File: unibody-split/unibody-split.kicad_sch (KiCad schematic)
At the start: 103 parts, among them IC1 AP130-20, SW1 SW_Push, SW10 SW_Push, SW11 SW_Push, SW12 SW_Push, SW13 SW_Push, SW14 SW_Push, SW15 SW_Push, SW16 SW_Push, SW17 SW_Push, SW18 SW_Push, SW19 SW_Push, SW2 SW_Push, SW20 SW_Push, SW21 SW_Push, SW22 SW_Push, SW23 SW_Push, SW24 SW_Push, SW25 SW_Push, SW26 SW_Push, SW27 SW_Push, SW28 SW_Push, SW29 SW_Push, SW3 SW_Push, SW30 SW_Push, SW31 SW_Push, SW32 SW_Push, SW33 SW_Push, SW34 SW_Push, SW35 SW_Push, SW36 SW_Push, SW37 SW_Push, SW38 SW_Push, SW39 SW_Push, SW4 SW_Push, SW40 SW_Push, SW41 SW_Push, SW42 SW_Push, SW5 SW_Push, SW6 SW_Push, SW7 SW_Push, SW8 SW_Push, SW9 SW_Push, U1 Pico, U2 PMW3360DM-T2QU, U3 HackPackv4-rescue:PSP_1000_JS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, U4 HackPackv4-rescue:PSP_1000_JS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, U5 HackPackv4-rescue:PSP_1000_JS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

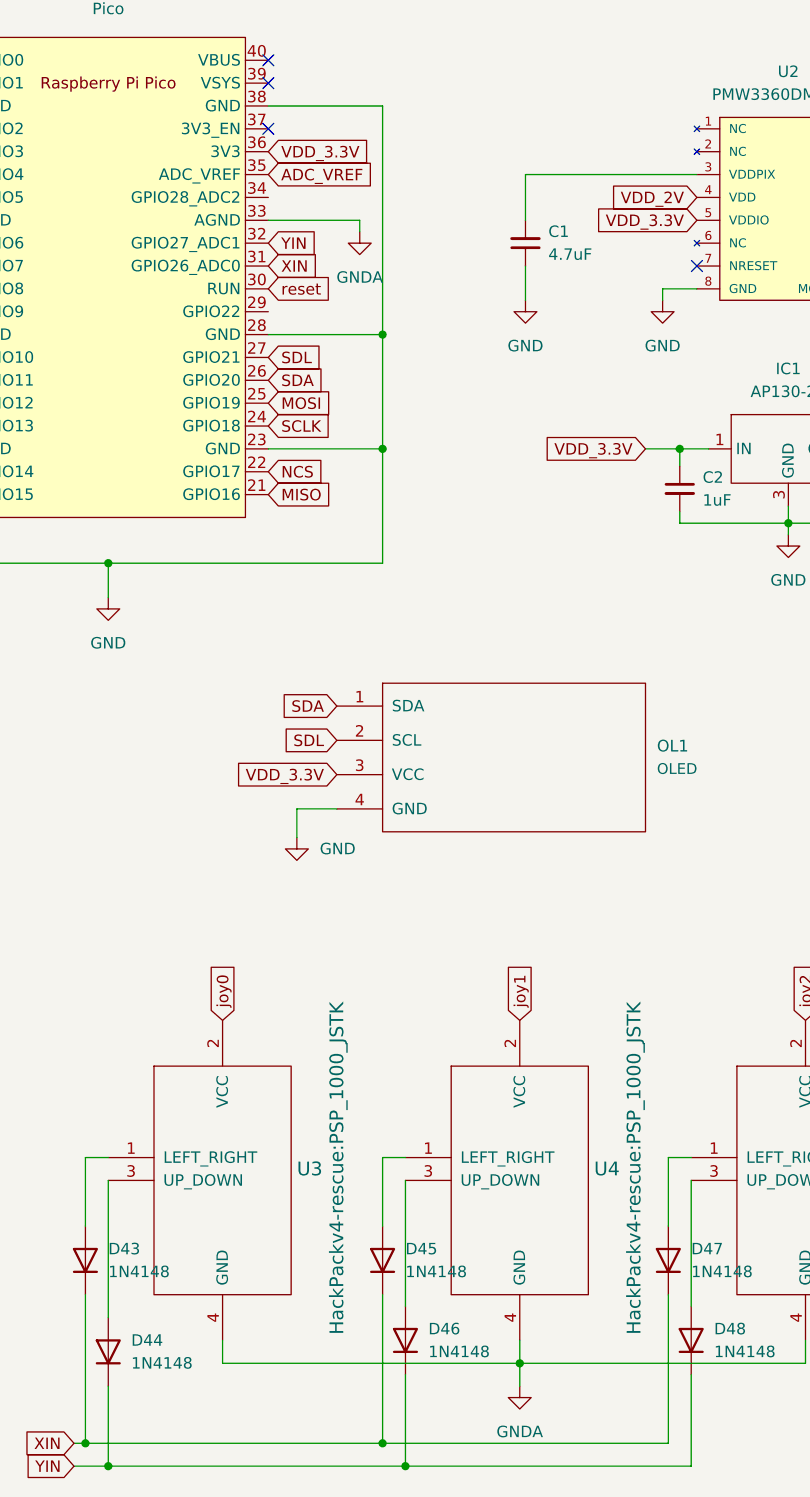
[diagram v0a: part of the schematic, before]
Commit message: Done routing PCB
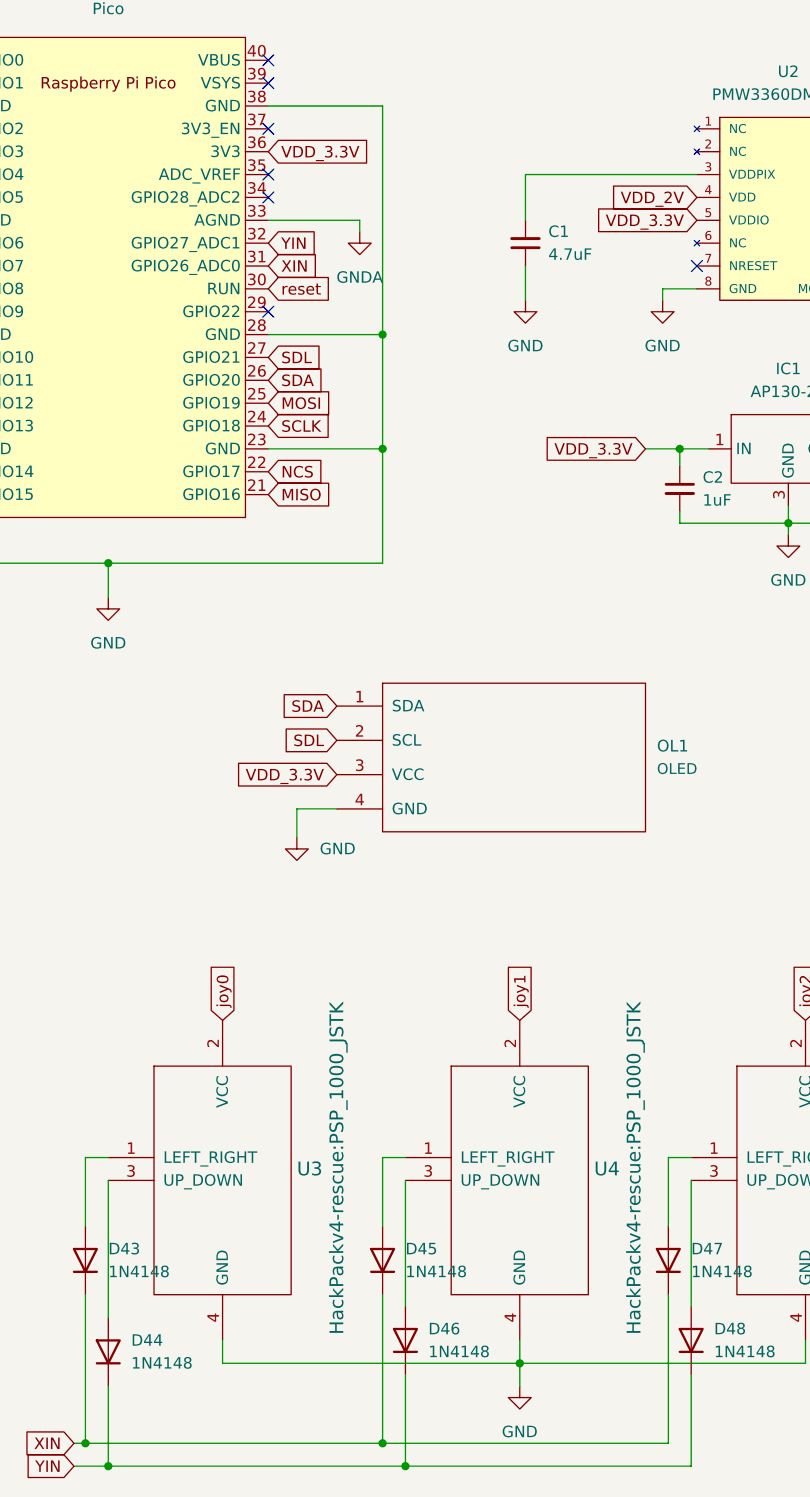
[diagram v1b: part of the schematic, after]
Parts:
- D1, D10, D11, D12, D13, D14, D15, D16, D17, D18, D19, D2, D20, D21, D22, D23, D24, D25, D26, D27, D28, D29, D3, D30, D31, D32, D33, D34, D35, D36, D37, D38, D39, D4, D40, D41, D42, D43, D44, D45, D46, D47, D48, D5, D6, D7, D8, D9: footprint Diode_THT:D_DO-35_SOD27_P7.62mm_Horizontal -> unibody-split:D_DO-35_SOD27_P7.62mm_Horizontal
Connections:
- net GND: now also U3.4 (GND), U4.4 (GND), U5.4 (GND)
- net GNDA: no longer U3.4 (GND), U4.4 (GND), U5.4 (GND)
- net ADC_VREF: no longer names the net of U1.35 (ADC_VREF)
- no-connect marks 5 -> 8
